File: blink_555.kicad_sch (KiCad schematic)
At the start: 8 parts, among them J1 PWR, U1 NE555P

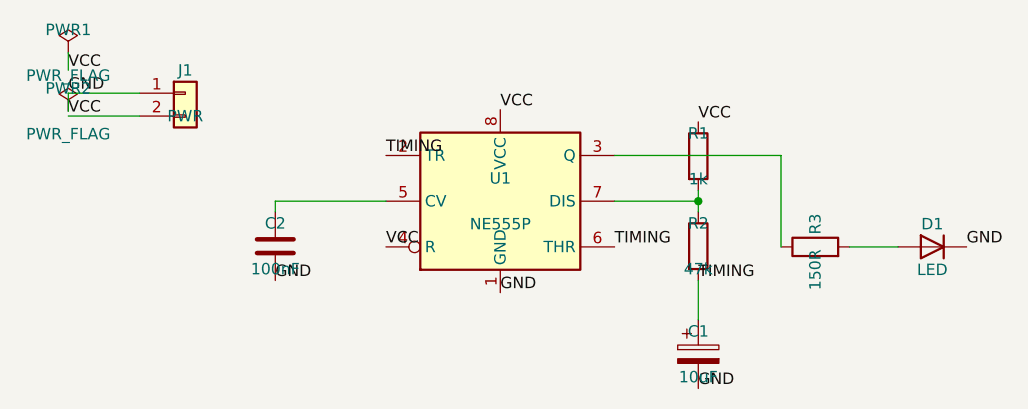
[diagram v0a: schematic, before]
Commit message: working on pcb
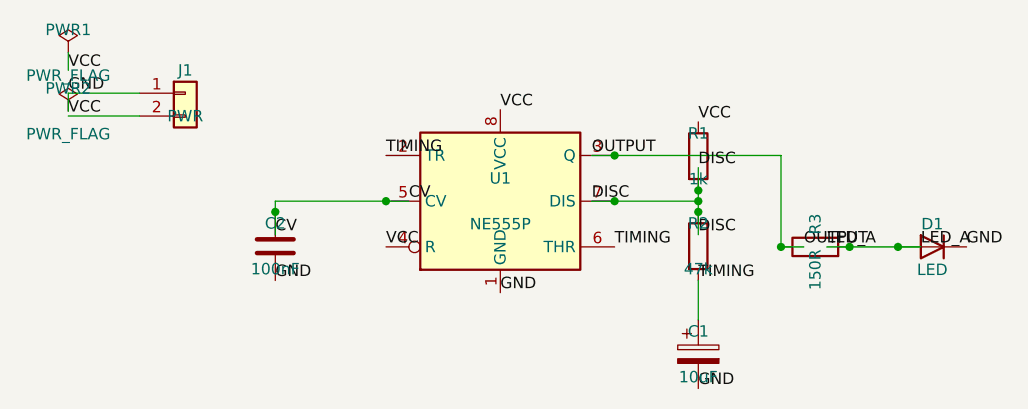
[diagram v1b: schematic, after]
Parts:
- C1: footprint (none) -> Capacitor_SMD:CP_Elec_5x5.4; LCSC (none) -> C72487
- C2: footprint (none) -> Capacitor_SMD:C_0603_1608Metric; LCSC (none) -> C14663
- D1: footprint (none) -> LED_SMD:LED_0805_2012Metric; LCSC (none) -> C84256
- J1: footprint (none) -> Connector_PinHeader_2.54mm:PinHeader_1x02_P2.54mm_Vertical; LCSC (none) -> C492401
- R1: footprint (none) -> Resistor_SMD:R_0603_1608Metric; LCSC (none) -> C21190
- R2: footprint (none) -> Resistor_SMD:R_0603_1608Metric; LCSC (none) -> C25819
- R3: footprint (none) -> Resistor_SMD:R_0603_1608Metric; LCSC (none) -> C22808
- U1: footprint (none) -> Package_DIP:DIP-8_W7.62mm; LCSC (none) -> C19708138
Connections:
- net DISC: now reaches R1.2, R2.1, U1.7 (DIS)
- net CV: now reaches C2.1, U1.5 (CV)
- net OUTPUT: now reaches R3.1, U1.3 (Q)
- net LED_A: now reaches D1.2 (A), R3.2
